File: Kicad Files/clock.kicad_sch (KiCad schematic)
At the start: 28 parts, among them SW1 SW_Push, SW2 SW_SPDT, U4 NE555P, U5 NE555P, U6 74HC04, U7 74HC00, U8 NE555P

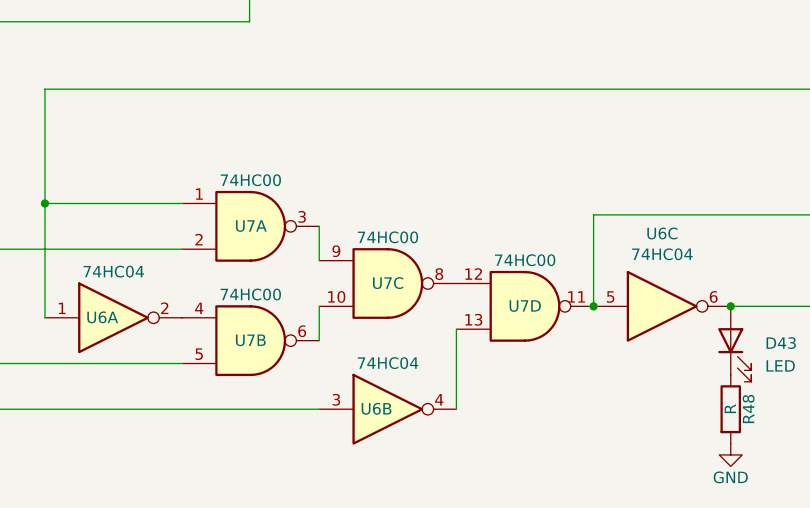
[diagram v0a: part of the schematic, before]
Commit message: update
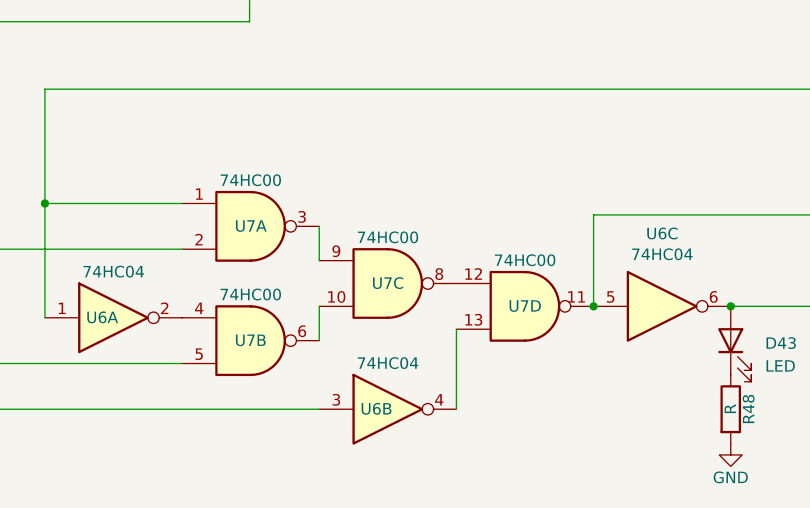
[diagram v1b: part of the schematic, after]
